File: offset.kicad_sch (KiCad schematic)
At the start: 32 parts, among them U11 OPA2189DGK, U12 TMUX1108PW, U19 TCA0372

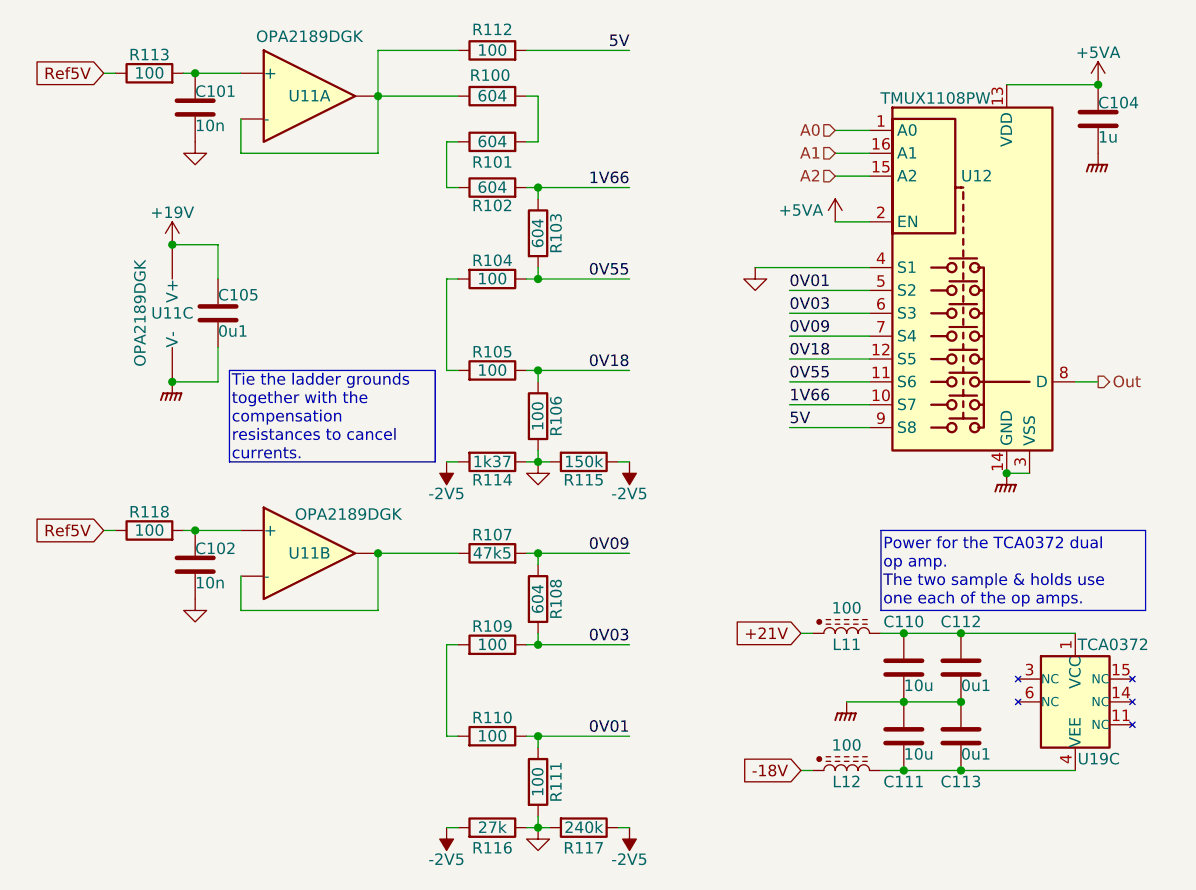
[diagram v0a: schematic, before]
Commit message: Progress checkin.  About to redo FDA feedback again.
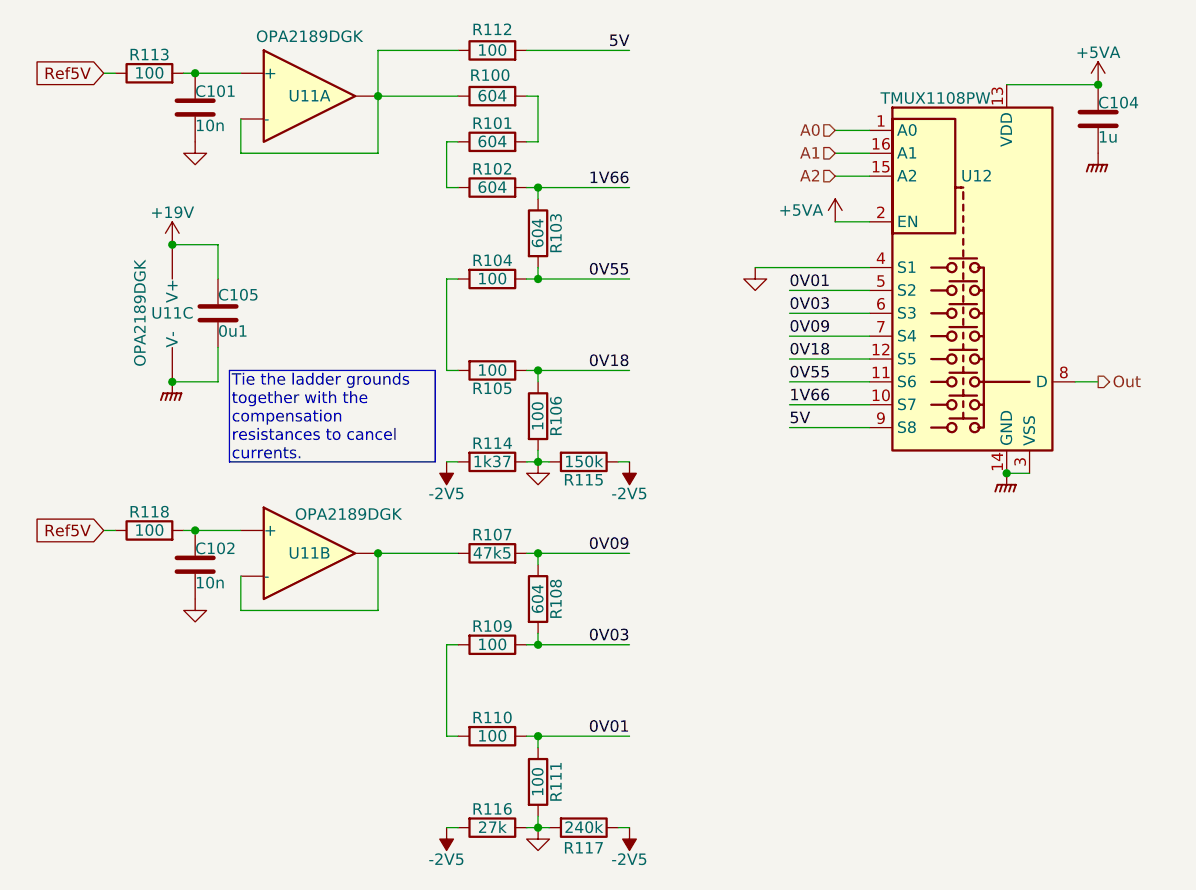
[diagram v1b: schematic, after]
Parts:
- removed C110, C111: 10u, Capacitor_SMD:C_0805_2012Metric, symbol Device:C
- removed C112, C113: 0u1, Capacitor_SMD:C_0402_1005Metric, symbol Device:C
- removed L11, L12: 100, Inductor_SMD:L_0603_1608Metric, symbol Parts:L_Ferrite_Power
- removed U19: TCA0372, Package_SO:SOIC-16W_7.5x10.3mm_P1.27mm, symbol Parts:TCA0372
